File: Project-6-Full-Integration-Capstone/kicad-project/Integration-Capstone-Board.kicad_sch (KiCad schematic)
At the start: 42 parts, among them J1 Conn_01x02, J2 Conn_01x02, J3 Conn_01x02, J4 Conn_01x04, J5 Conn_01x07, J6 Conn_01x04, J7 Conn_01x12, J8 Conn_01x04, J9 USB_B_Micro, SW1 SW_SPST, U1 AMS1117-3.3, U2 STM32F411RETx, U3 USBLC6-2SC6, Y1 Crystal

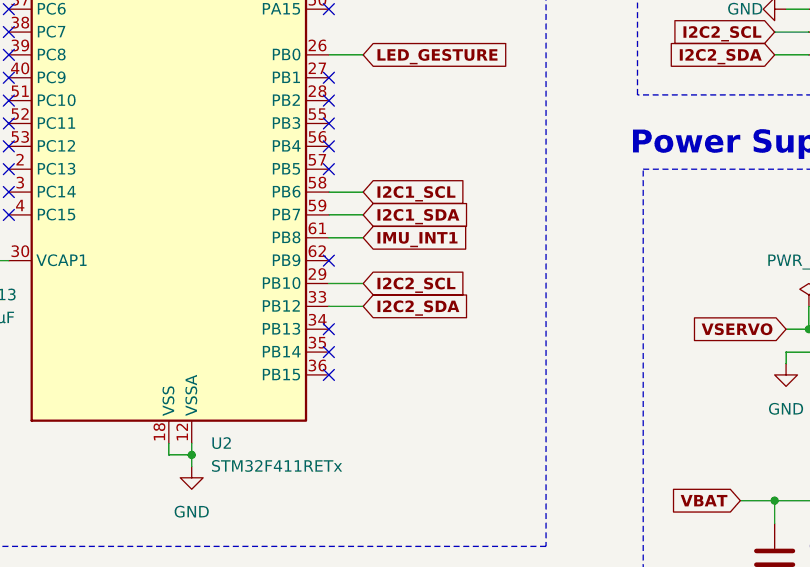
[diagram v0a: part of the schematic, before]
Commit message: Integration-Capstone-Board-Update
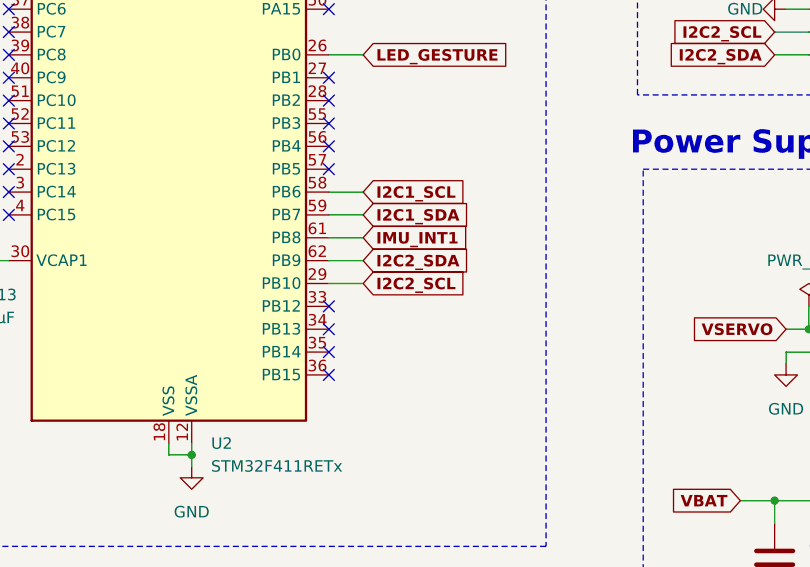
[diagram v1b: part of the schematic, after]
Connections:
- net I2C2_SDA: now also U2.62 (PB9); no longer U2.33 (PB12)
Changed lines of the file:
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@@
+	)
+	(no_connect
+		(at 124.46 119.38)
 	)
 	(no_connect
@@
 	)
 	(no_connect
-		(at 124.46 114.3)
-	)
-	(no_connect
 		(at 124.46 83.82)
 	)
@@
 	(wire
 		(pts
-			(xy 124.46 119.38) (xy 128.27 119.38)
-		)
-		(stroke
-			(width 0)
-			(type default)
-		)
-	)
-	(wire
-		(pts
 			(xy 82.55 49.53) (xy 85.09 49.53)
 		)
@@
 	(wire
 		(pts
+			(xy 124.46 114.3) (xy 128.27 114.3)
+		)
+		(stroke
+			(width 0)
+			(type default)
+		)
+	)
+	(wire
+		(pts
 			(xy 173.99 91.44) (xy 177.8 91.44)
 		)
@@
 		)
 	)
+	(global_label "I2C2_SDA"
+		(shape input)
+		(at 128.27 114.3 0)
+		(fields_autoplaced yes)
+		(effects
+			(font
+				(size 1.27 1.27)
+				(thickness 0.254)
+				(bold yes)
+			)
+			(justify left)
+		)
+		(property "Intersheetrefs" "${INTERSHEET_REFS}"
+			(at 140.5607 114.3 0)
+			(effects
+				(font
+					(size 1.27 1.27)
+				)
+				(justify left)
+				(hide yes)
+			)
+		)
+	)
 	(global_label "I2C1_SDA"
 		(shape input)
@@
 				(hide yes)
 			)
-		)
-	)
-	(global_label "I2C2_SDA"
-		(shape input)
-		(at 128.27 119.38 0)
-		(fields_autoplaced yes)
-		(effects
-			(font
-				(size 1.27 1.27)
-				(thickness 0.254)
-				(bold yes)
-			)
-			(justify left)
-		)
-		(property "Intersheetrefs" "${INTERSHEET_REFS}"
-			(at 140.5607 119.38 0)
-			(effects
-				(font
-					(size 1.27 1.27)
-				)
-				(justify left)
-				(hide yes)
-			)
